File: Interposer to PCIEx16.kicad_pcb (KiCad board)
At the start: 2 copper layers, 38.1 x 17.1 mm, 19 parts, among them U1 BuckBoostIC, U3 5v_Regulator, U4 +12V, U5 VIN, U6 GND

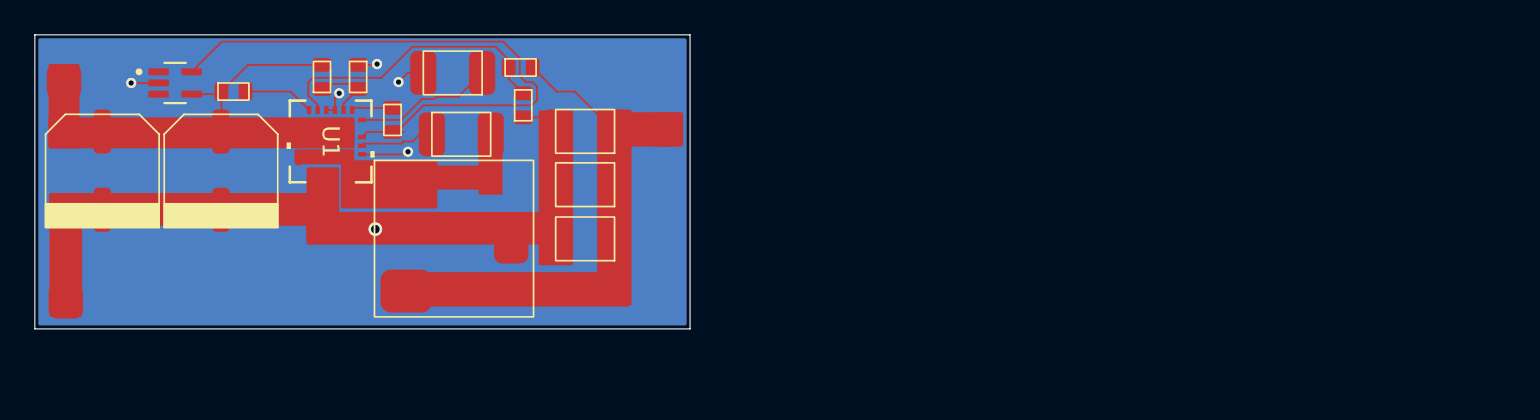
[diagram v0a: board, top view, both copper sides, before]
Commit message: Add files via upload
V0.2
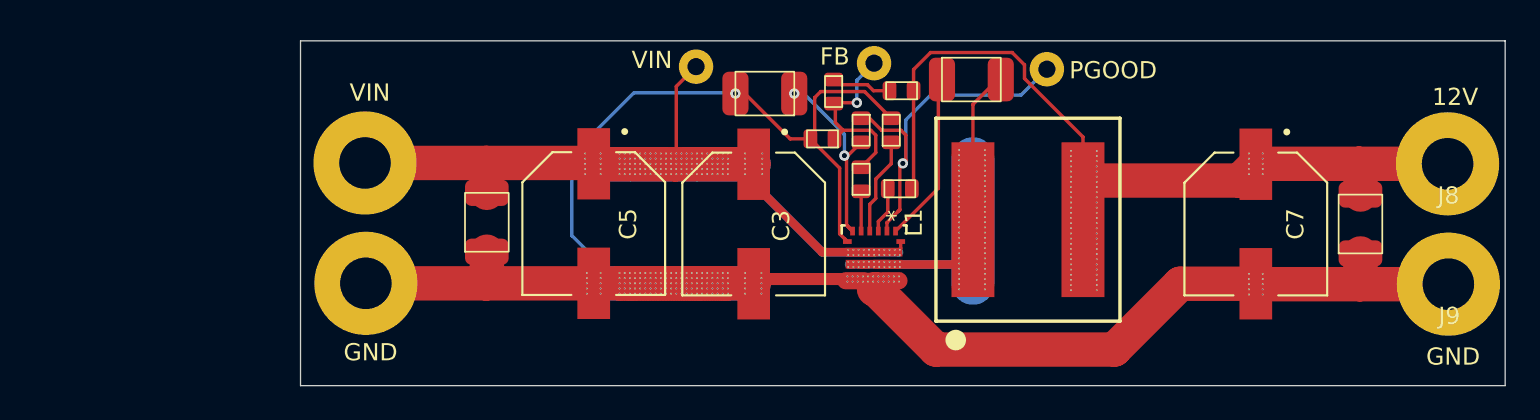
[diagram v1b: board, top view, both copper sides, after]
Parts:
- removed R11: 10k, FW 16 Components:0603
- removed U1: BuckBoostIC, FW 16 Components:BuckBoostIC
- removed U4: +12V, FW 16 Components:PAD
- removed U5: VIN, FW 16 Components:PAD
- removed U6: GND, FW 16 Components:PAD
- added J3: ~, FW 16 Components:TestPad, F.Cu at (101.5, 20.4)
- added J4: ~, FW 16 Components:TestPad, F.Cu at (91.4, 20.1)
- added J5: ~, FW 16 Components:TestPad, F.Cu at (81.0, 20.2)
- added J6: ~, FW 16 Components:PowerTHT, F.Cu at (61.9, 28.2)
- added J7: ~, FW 16 Components:PowerTHT, F.Cu at (61.9, 35.2)
- added J8: ~, FW 16 Components:PowerTHT, F.Cu at (124.8, 28.2)
- added J9: ~, FW 16 Components:PowerTHT, F.Cu at (124.8, 35.2)
- added R12: 10k, FW 16 Components:0603, F.Cu at (92.4, 24.0)
- added R13: 10, FW 16 Components:0603, F.Cu at (90.7, 26.9)
- C1: value 22uf -> 1.0uf; footprint FW 16 Components:22uf 25V -> FW 16 Components:1210 capacitor
- C3, C5: value ~ -> 100uf; footprint FW 16 Components:1210 capacitor -> FW 16 Components:25SVPF100M
- C4: value ~ -> .1uf
- C6: value .01uf -> .1uf
- C7: value 22uf -> 100uf; footprint FW 16 Components:22uf 25V -> FW 16 Components:25SVPF100M
- L1: value ~ -> WE-XHMA_1090; footprint FW 16 Components:3.3uH -> FW 16 Components:WE-XHMA_1090
- R10: value 10k -> 10
- R6: value 200k -> 47.5k
- R7: value 10k -> 100k
- R8: value 30k -> 10k
- R9: value 140k -> 10k
- U3: value 5v_Regulator -> BD9F800MUX-ZE2; footprint FW 16 Components:5v Regulator -> FW 16 Components:VQFN11_ROM
- moved C7 56.8 mm to (113.6, 29.4), turned to -90 degrees
- moved C6 56.6 mm to (122.2, 29.2), turned to 90 degrees
- moved U3 41.9 mm to (91.4, 31.4), turned to -90 degrees
- moved R6 39.0 mm to (93.0, 21.6), turned to 180 degrees
- moved C1 35.6 mm to (84.9, 19.3), turned to 180 degrees
- moved L1 33.6 mm to (100.3, 29.1), turned to 90 degrees
- moved C2 29.8 mm to (97.2, 23.5)
- moved R8 29.4 mm to (88.5, 24.4), turned to 180 degrees
- moved R7 27.7 mm to (89.0, 21.6)
- moved R10 22.4 mm to (92.8, 27.4), turned to 0 degrees
- moved R9 20.2 mm to (90.7, 23.9), turned to -90 degrees
- moved C3 11.0 mm to (84.4, 29.4), turned to -90 degrees
- moved C4 8.21 mm to (71.4, 29.1), turned to 90 degrees
- moved C5 1.74 mm to (75.1, 29.4), turned to -90 degrees
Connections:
- net EN renamed Net-(J4-Pad1)
- C1 pad 1: GND -> VREG
- C1 pad 2: VIN -> GND
- C2 pad 1: Net-(U1-BST) -> Net-(U3-BOOT)
- C2 pad 2: LX -> SW
- C3 pad 1: +12V -> VIN
- C4 pad 1: +12V -> GND
- C4 pad 2: GND -> VIN
- C5 pad 1: +12V -> VIN
- C6 pad 1: Net-(U1-SS) -> GND
- C6 pad 2: GND -> +12V
- C7 pad 1: GND -> +12V
- C7 pad 2: VIN -> GND
- L1 pad 1: +12V -> SW
- L1 pad 2: LX -> +12V
- R10 pad 1: GND -> Net-(U3-VOUT)
- R10 pad 2: FB -> +12V
- R6 pad 1: VIN -> +12V
- R6 pad 2: Net-(U1-TON) -> Net-(R6-Pad2)
- R7 pad 1: GND -> Net-(R6-Pad2)
- R8 pad 2: VIN -> GND
- R9 pad 1: FB -> Net-(U3-PGD)
- R9 pad 2: +12V -> VREG
- U3 pad 1: (no net) -> Net-(U3-BOOT)
- U3 pad 2: GND -> Net-(U3-PGD)
- U3 pad 3: (no net) -> Net-(U3-VOUT)
- U3 pad 4: VIN -> Net-(U3-FREQ)
- U3 pad 5: +5V -> Net-(U3-FB)
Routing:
- net GND: track 16.2 -> 134.6 mm, vias 6 -> 163
- net VIN: track 10.6 -> 104.4 mm, vias 0 -> 152
- net +12V: track 6.30 -> 48.4 mm, vias 0 -> 66
- net SW: track 0.00 -> 39.1 mm, vias 0 -> 78
- net +5V: track 35.6 -> 0.00 mm
- net Net-(U3-PGD): track 0.00 -> 21.2 mm, vias 0 -> 1
- net FB: track 17.0 -> 0.00 mm
- net VREG: track 0.00 -> 12.3 mm, vias 0 -> 2
- net Net-(U3-BOOT): track 0.00 -> 9.81 mm
- net Net-(U1-SS): track 8.12 -> 0.00 mm
- net Net-(J4-Pad1): track 3.93 -> 10.7 mm, vias 0 -> 1
- net Net-(U3-FREQ): track 0.00 -> 5.68 mm
- net Net-(U1-TON): track 4.36 -> 0.00 mm
- net Net-(U1-BST): track 4.06 -> 0.00 mm
- net Net-(R6-Pad2): track 0.00 -> 3.37 mm
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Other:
- board size 38.1 x 17.1 mm -> 70 x 20 mm
- board text added: "12V"
- board text added: "FB"
- board text added: "GND"
- board text added: "PGOOD"
- board text added: "VIN"
